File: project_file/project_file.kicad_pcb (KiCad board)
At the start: 2 copper layers, 44 x 84 mm, 76 parts, among them IC1 BMI055, J1 Power Module 1, J10 CAP & ADC IN, J11 SPI Port, J12 I2C A, J13 FMU PWM OUT, J14 PPM RC, J15 2908-05WB-MG, J16 RC, J17 SBUS, J18 IO/PWM out, J2 Power Module 2, J3 USB, J4 Telemetry 1, J5 Telemetry 2, J6 UART & I2C B, J7 CAN 1, J8 CAN 2, J9 GPS Module, U1 STM32F765IIKx, U10 TJA1051TK-3, U11 LT3080xDD, U12 LP5907MFX-3.3, U13 LP5907MFX-3.3, U3 IST8310, U4 ICM-20602, U5 ICM-20689, U6 MS5611-01BA, U8 STM32F103V8Tx, U9 TJA1051TK-3, Y1 ABM2-8.000MHZ-D4Y-T

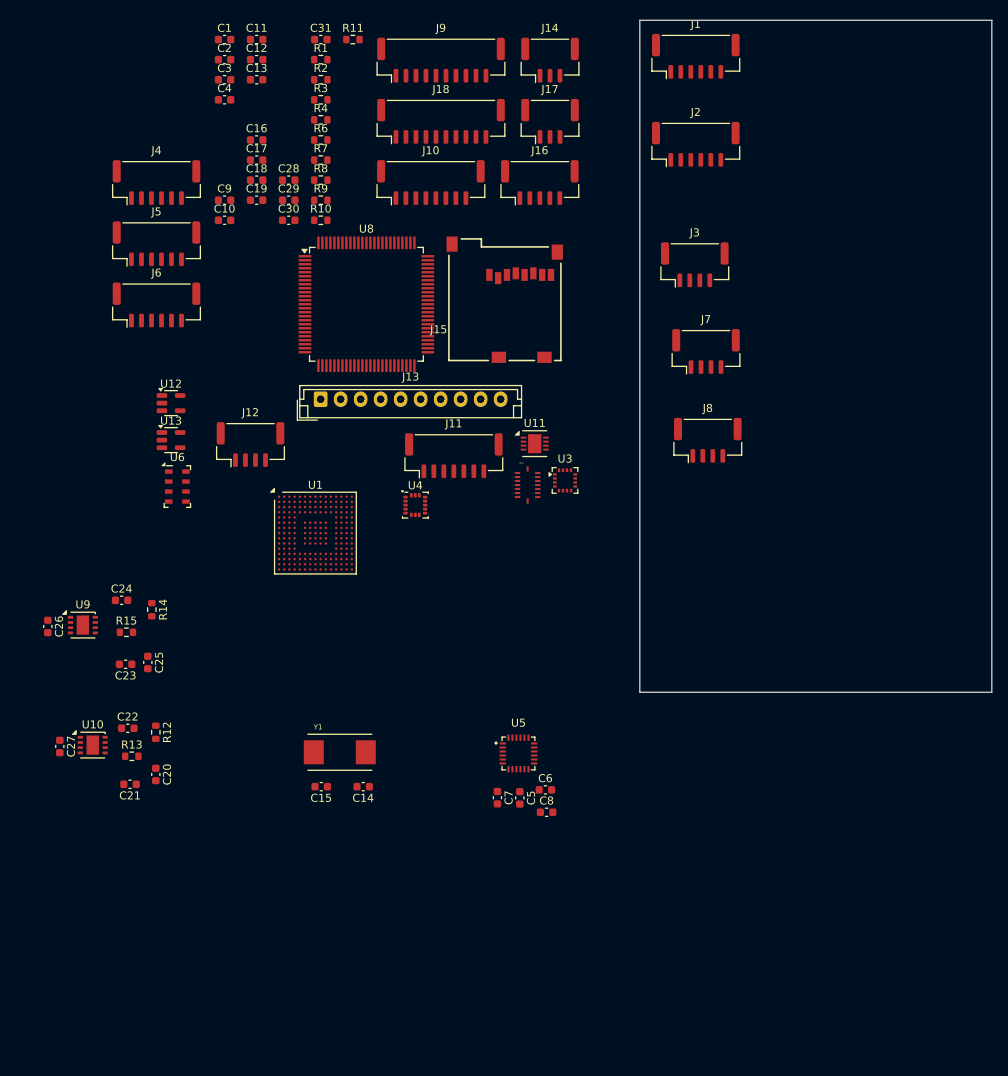
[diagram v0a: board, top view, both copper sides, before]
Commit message: more grouping
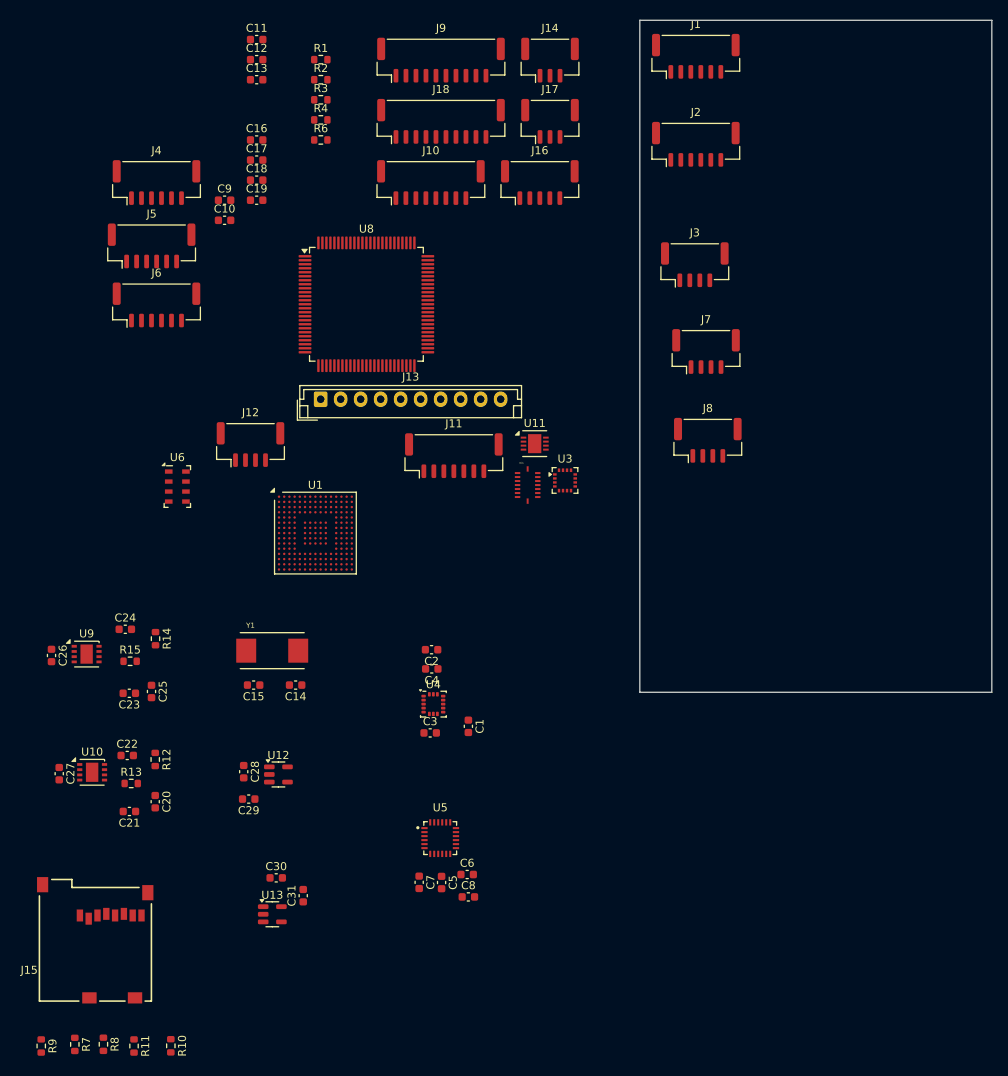
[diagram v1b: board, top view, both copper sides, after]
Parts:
- moved R11 128.7 mm to (43.8, 158.2), turned to -90 degrees
- moved R7 114.7 mm to (36.4, 158.0), turned to -90 degrees
- moved R8 111.4 mm to (40.0, 158.0), turned to -90 degrees
- moved R9 111.4 mm to (32.2, 158.2), turned to -90 degrees
- moved C31 107.0 mm to (64.9, 139.4), turned to 90 degrees
- moved R10 104.9 mm to (48.4, 158.2), turned to -90 degrees
- moved J15 95.0 mm to (39.0, 145.0)
- moved C1 91.1 mm to (85.6, 118.3), turned to -90 degrees
- moved C3 85.6 mm to (80.8, 119.1)
- moved C30 82.2 mm to (61.5, 137.2)
- moved C2 78.2 mm to (81.0, 108.7), turned to 180 degrees
- moved C4 75.7 mm to (81.0, 111.1), turned to 180 degrees
- moved C29 75.0 mm to (58.1, 127.3), turned to 180 degrees
- moved C28 74.2 mm to (57.5, 123.9), turned to -90 degrees
- moved U13 60.6 mm to (61.1, 141.8)
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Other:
- board text added: "3V3 REG"
- board text added: "5V REG"
- board text added: "ICM-20602"
- board text added: "MICRO SD"
